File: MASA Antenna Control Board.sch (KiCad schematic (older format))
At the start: 32 parts, among them J1 UJ2-MBH-1-SMT, J2 Conn_01x06_Male, J3 Conn_01x02_Male, J4 Conn_01x02_Male, J5 Conn_01x04_Male, U1 BL654PA, U2 XBP9B-DPST-001, U3 XBP9B-DPST-001, U4 XBP9B-DPST-001, U5 TPS563200

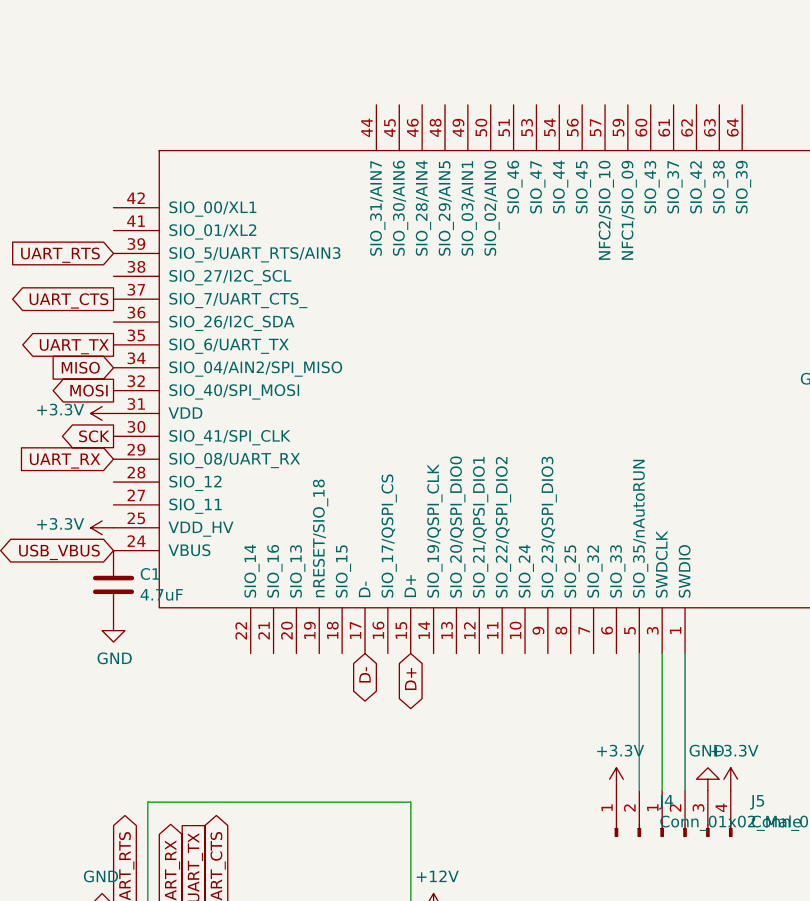
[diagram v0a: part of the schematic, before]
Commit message: Finished most routing
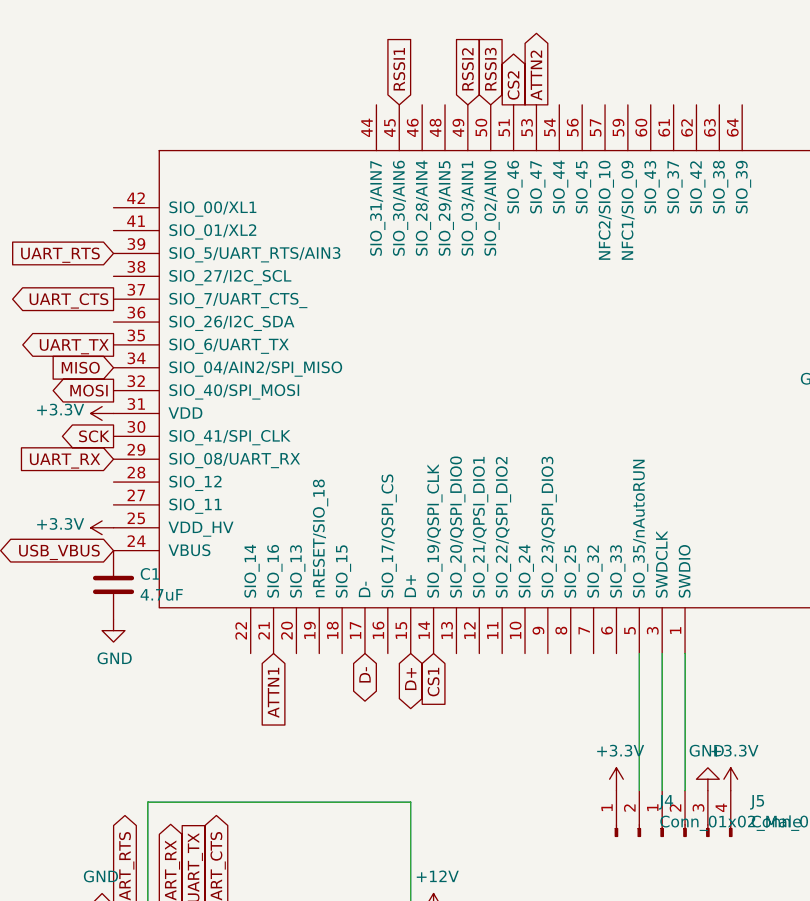
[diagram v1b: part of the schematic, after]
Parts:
- C14, C15, C5: footprint Capacitor_THT:CP_Axial_L11.0mm_D5.0mm_P18.00mm_Horizontal -> Capacitor_THT:CP_Radial_D5.0mm_P2.00mm
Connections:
- net ATTN1: now also U1.21 (SIO_16)
- net ATTN2: now also U1.53 (SIO_47)
- net CS1: now also U1.14 (SIO_19/QSPI_CLK)
- net CS2: now also U1.51 (SIO_46)
- net RSSI1: now also U1.45 (SIO_30/AIN6)
- net RSSI2: now also U1.49 (SIO_03/AIN1)
- net RSSI3: now also U1.50 (SIO_02/AIN0)
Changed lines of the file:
@@
 F 0 "C15" H 10818 2396 50  0000 L CNN
 F 1 "10μF" H 10818 2305 50  0000 L CNN
-F 2 "Capacitor_THT:CP_Axial_L11.0mm_D5.0mm_P18.00mm_Horizontal" H 10738 2200 50  0001 C CNN
+F 2 "Capacitor_THT:CP_Radial_D5.0mm_P2.00mm" H 10738 2200 50  0001 C CNN
 F 3 "~" H 10700 2350 50  0001 C CNN
 	1    10700 2350
@@
 F 0 "C14" H 10368 2396 50  0000 L CNN
 F 1 "10μF" H 10368 2305 50  0000 L CNN
-F 2 "Capacitor_THT:CP_Axial_L11.0mm_D5.0mm_P18.00mm_Horizontal" H 10288 2200 50  0001 C CNN
+F 2 "Capacitor_THT:CP_Radial_D5.0mm_P2.00mm" H 10288 2200 50  0001 C CNN
 F 3 "~" H 10250 2350 50  0001 C CNN
 	1    10250 2350
@@
 F 0 "C5" H 7118 2646 50  0000 L CNN
 F 1 "22μF" H 7118 2555 50  0000 L CNN
-F 2 "Capacitor_THT:CP_Axial_L11.0mm_D5.0mm_P18.00mm_Horizontal" H 7038 2450 50  0001 C CNN
+F 2 "Capacitor_THT:CP_Radial_D5.0mm_P2.00mm" H 7038 2450 50  0001 C CNN
 F 3 "~" H 7000 2600 50  0001 C CNN
 	1    7000 2600
@@
 	0    -1   -1   0
 $EndComp
+Text GLabel 3100 1150 1    50   Input ~ 0
+RSSI2
+Text GLabel 2800 1150 1    50   Input ~ 0
+RSSI1
+Text GLabel 3200 1150 1    50   Input ~ 0
+RSSI3
+Text GLabel 3300 1150 1    50   Output ~ 0
+CS2
+Text GLabel 3400 1150 1    50   Output ~ 0
+ATTN2
+Text GLabel 2250 3550 3    50   Input ~ 0
+ATTN1
+Text GLabel 2950 3550 3    50   Input ~ 0
+CS1
 $EndSCHEMATC
